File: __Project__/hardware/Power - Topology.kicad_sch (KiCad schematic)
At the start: 0 parts

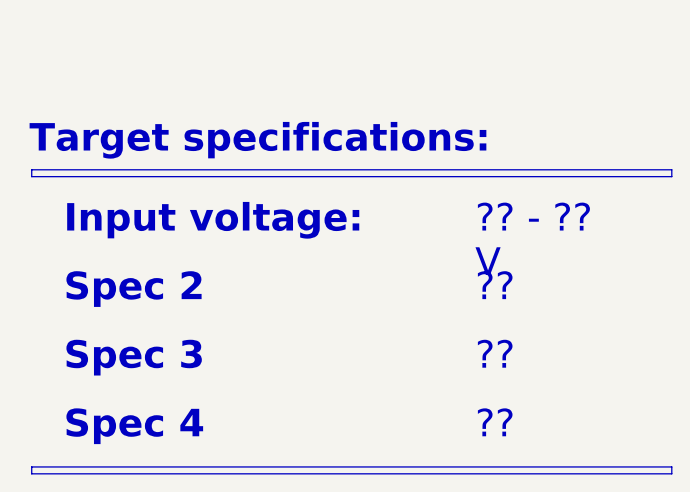
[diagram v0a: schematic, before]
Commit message: Update project template
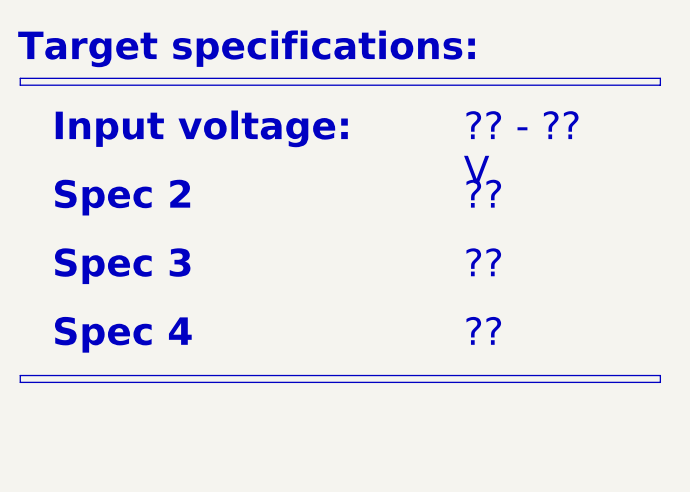
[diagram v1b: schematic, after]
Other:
- company: (none) -> ${COMPANY}
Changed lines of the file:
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@@
 	(generator_version "9.0")
 	(paper "A3")
+	(title_block
+		(date "2025-06-05")
+		(rev "${REVISION}")
+		(company "${COMPANY}")
+	)
 	(rectangle
-		(start 335.28 250.19)
-		(end 406.4 250.952)
+		(start 334.01 240.03)
+		(end 405.13 240.792)
 		(stroke
 			(width 0)
@@
 	)
 	(rectangle
-		(start 335.28 217.17)
-		(end 406.4 217.932)
+		(start 334.01 207.01)
+		(end 405.13 207.772)
 		(stroke
 			(width 0)
@@
 	(text_box "Spec 2"
 		(exclude_from_sim no)
-		(at 336.55 226.06 0)
+		(at 335.28 215.9 0)
 		(size 43.18 7.62)
 		(margins 2.2859 2.2859 2.2859 2.2859)
@@
 	(text_box "Input voltage:"
 		(exclude_from_sim no)
-		(at 336.55 218.44 0)
+		(at 335.28 208.28 0)
 		(size 41.91 7.62)
 		(margins 2.2859 2.2859 2.2859 2.2859)
@@
 	(text_box "Spec 4"
 		(exclude_from_sim no)
-		(at 336.55 241.3 0)
+		(at 335.28 231.14 0)
 		(size 44.45 7.62)
 		(margins 2.2859 2.2859 2.2859 2.2859)
@@
 	(text_box "?? - ?? V"
 		(exclude_from_sim no)
-		(at 382.27 218.44 0)
+		(at 381 208.28 0)
 		(size 24.13 7.62)
 		(margins 2.2859 2.2859 2.2859 2.2859)
@@
 	(text_box "Target specifications:"
 		(exclude_from_sim no)
-		(at 332.74 209.55 0)
+		(at 331.47 199.39 0)
 		(size 73.66 7.62)
 		(margins 2.2859 2.2859 2.2859 2.2859)
@@
 	(text_box "??"
 		(exclude_from_sim no)
-		(at 382.27 241.3 0)
+		(at 381 231.14 0)
 		(size 24.13 7.62)
 		(margins 2.2859 2.2859 2.2859 2.2859)
@@
 	(text_box "??"
 		(exclude_from_sim no)
-		(at 382.27 233.68 0)
+		(at 381 223.52 0)
 		(size 24.13 7.62)
 		(margins 2.2859 2.2859 2.2859 2.2859)
@@
 	(text_box "Spec 3"
 		(exclude_from_sim no)
-		(at 336.55 233.68 0)
+		(at 335.28 223.52 0)
 		(size 41.91 7.62)
 		(margins 2.2859 2.2859 2.2859 2.2859)
@@
 	(text_box "??"
 		(exclude_from_sim no)
-		(at 382.27 226.06 0)
-		(size 24.13 7.62)
-		(margins 2.2859 2.2859 2.2859 2.2859)
+		(at 381 215.9 0)
+		(size 24.13 7.62)
+		(margins 2.2859 2.2859 2.2859 2.2859)
